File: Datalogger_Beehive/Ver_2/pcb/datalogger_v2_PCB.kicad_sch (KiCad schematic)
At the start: 75 parts, among them U1 DS18B20, U10 DS18B20, U11 DS18B20, U12 DS18B20, U13 DS18B20, U14 DS18B20, U15 DS18B20, U16 DS18B20, U17 DS18B20, U18 DS18B20, U19 DS18B20, U2 DS18B20, U20 DS18B20, U21 DS18B20, U22 DS18B20, U23 DS18B20, U24 DS18B20, U25 DS18B20, U26 DS18B20, U27 DS18B20, U28 DS18B20, U29 DS18B20, U3 DS18B20, U30 DS18B20, U31 DS18B20, U32 DS18B20, U33 DS18B20, U34 DS18B20, U35 DS18B20, U36 DS18B20, U37 DS18B20, U38 DS18B20, U39 DS18B20, U4 DS18B20, U40 DS18B20, U41 DS18B20, U42 DS18B20, U43 DS18B20, U44 DS18B20, U45 DS18B20, U46 DS18B20, U47 DS18B20, U48 DS18B20, U49 DS18B20, U5 DS18B20, U50 DS18B20, U51 DS18B20, U52 DS18B20, U53 DS18B20, U54 DS18B20, U55 DS18B20, U56 DS18B20, U57 DS18B20, U58 DS18B20, U59 DS18B20, U6 DS18B20, U60 DS18B20, U61 DS18B20, U62 DS18B20, U63 DS18B20, U64 DS18B20, U65 DS18B20, U66 DS18B20, U67 DS18B20, U68 DS18B20, U69 DS18B20, U7 DS18B20, U70 DS18B20, U8 DS18B20, U9 DS18B20

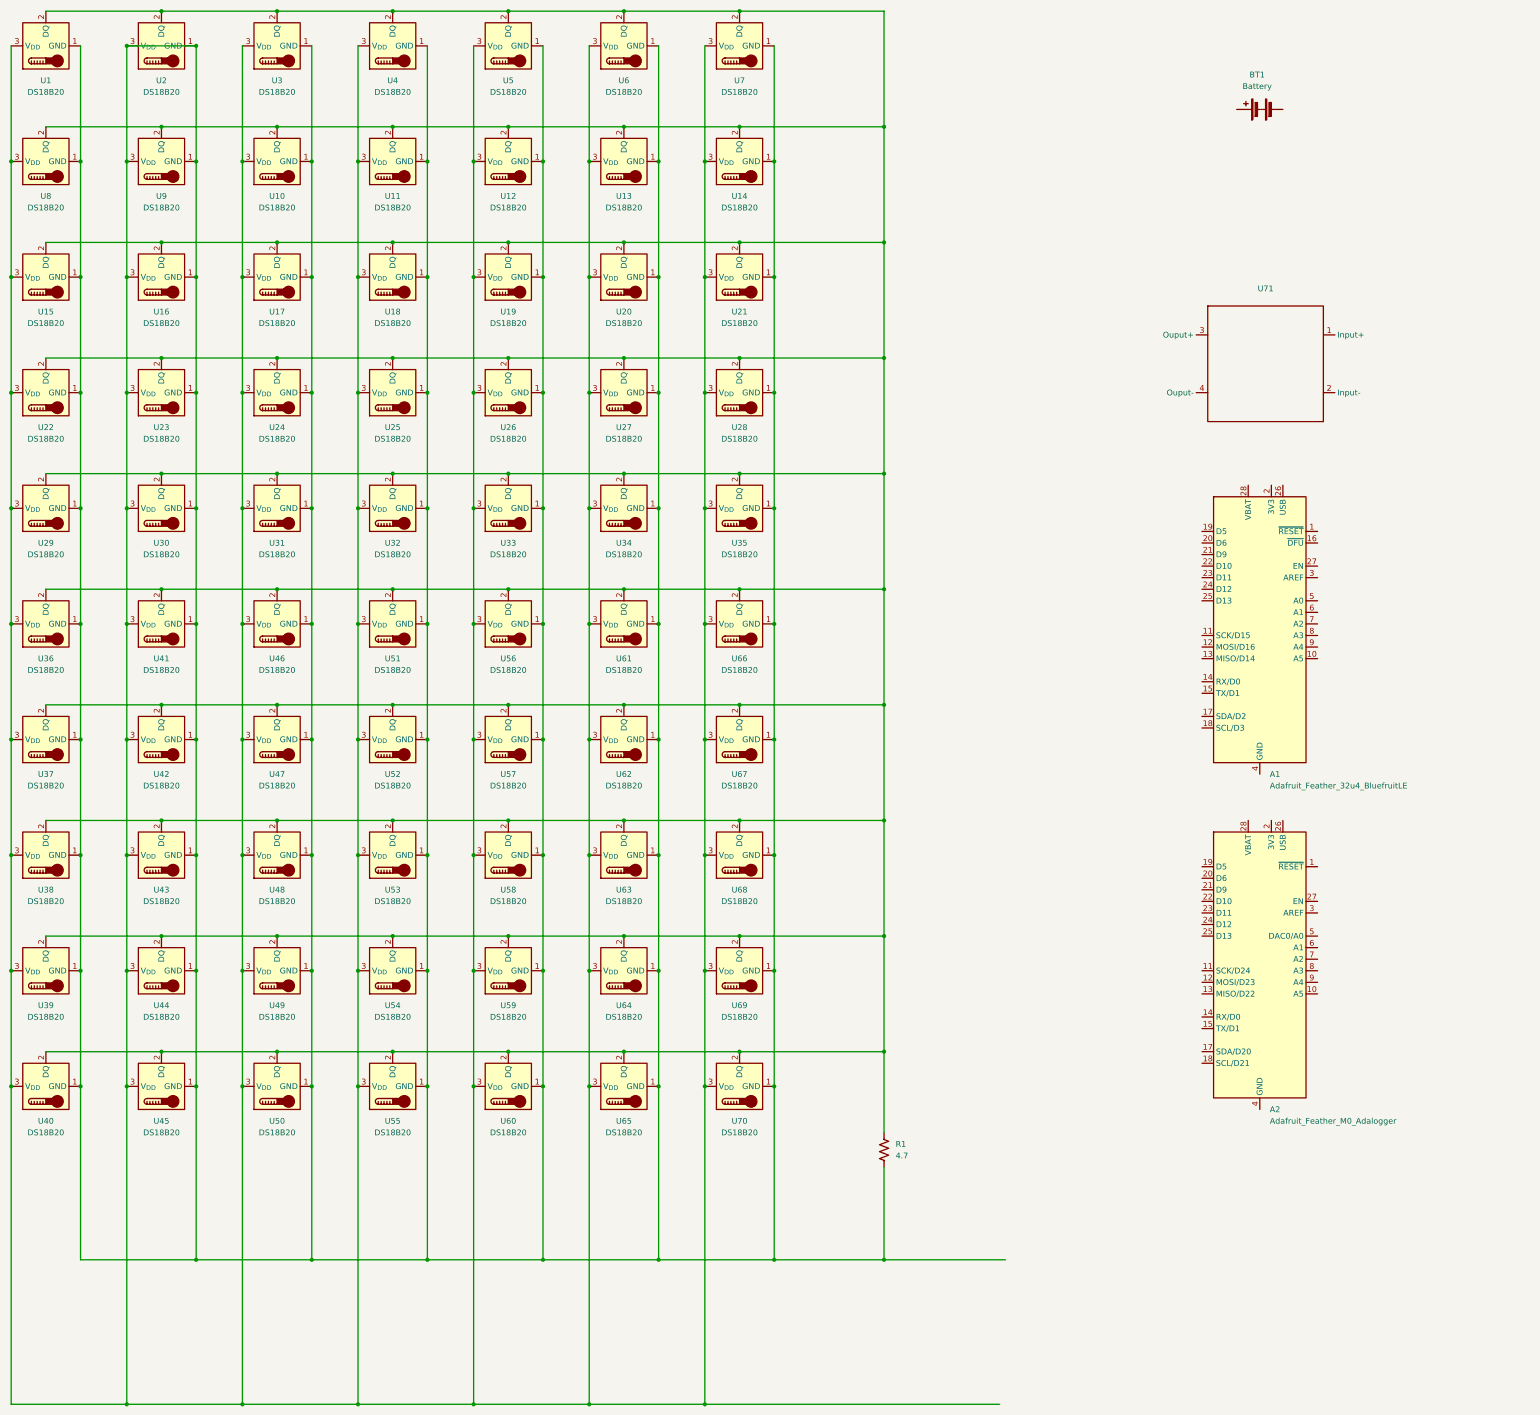
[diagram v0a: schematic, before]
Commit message: enclosure adding
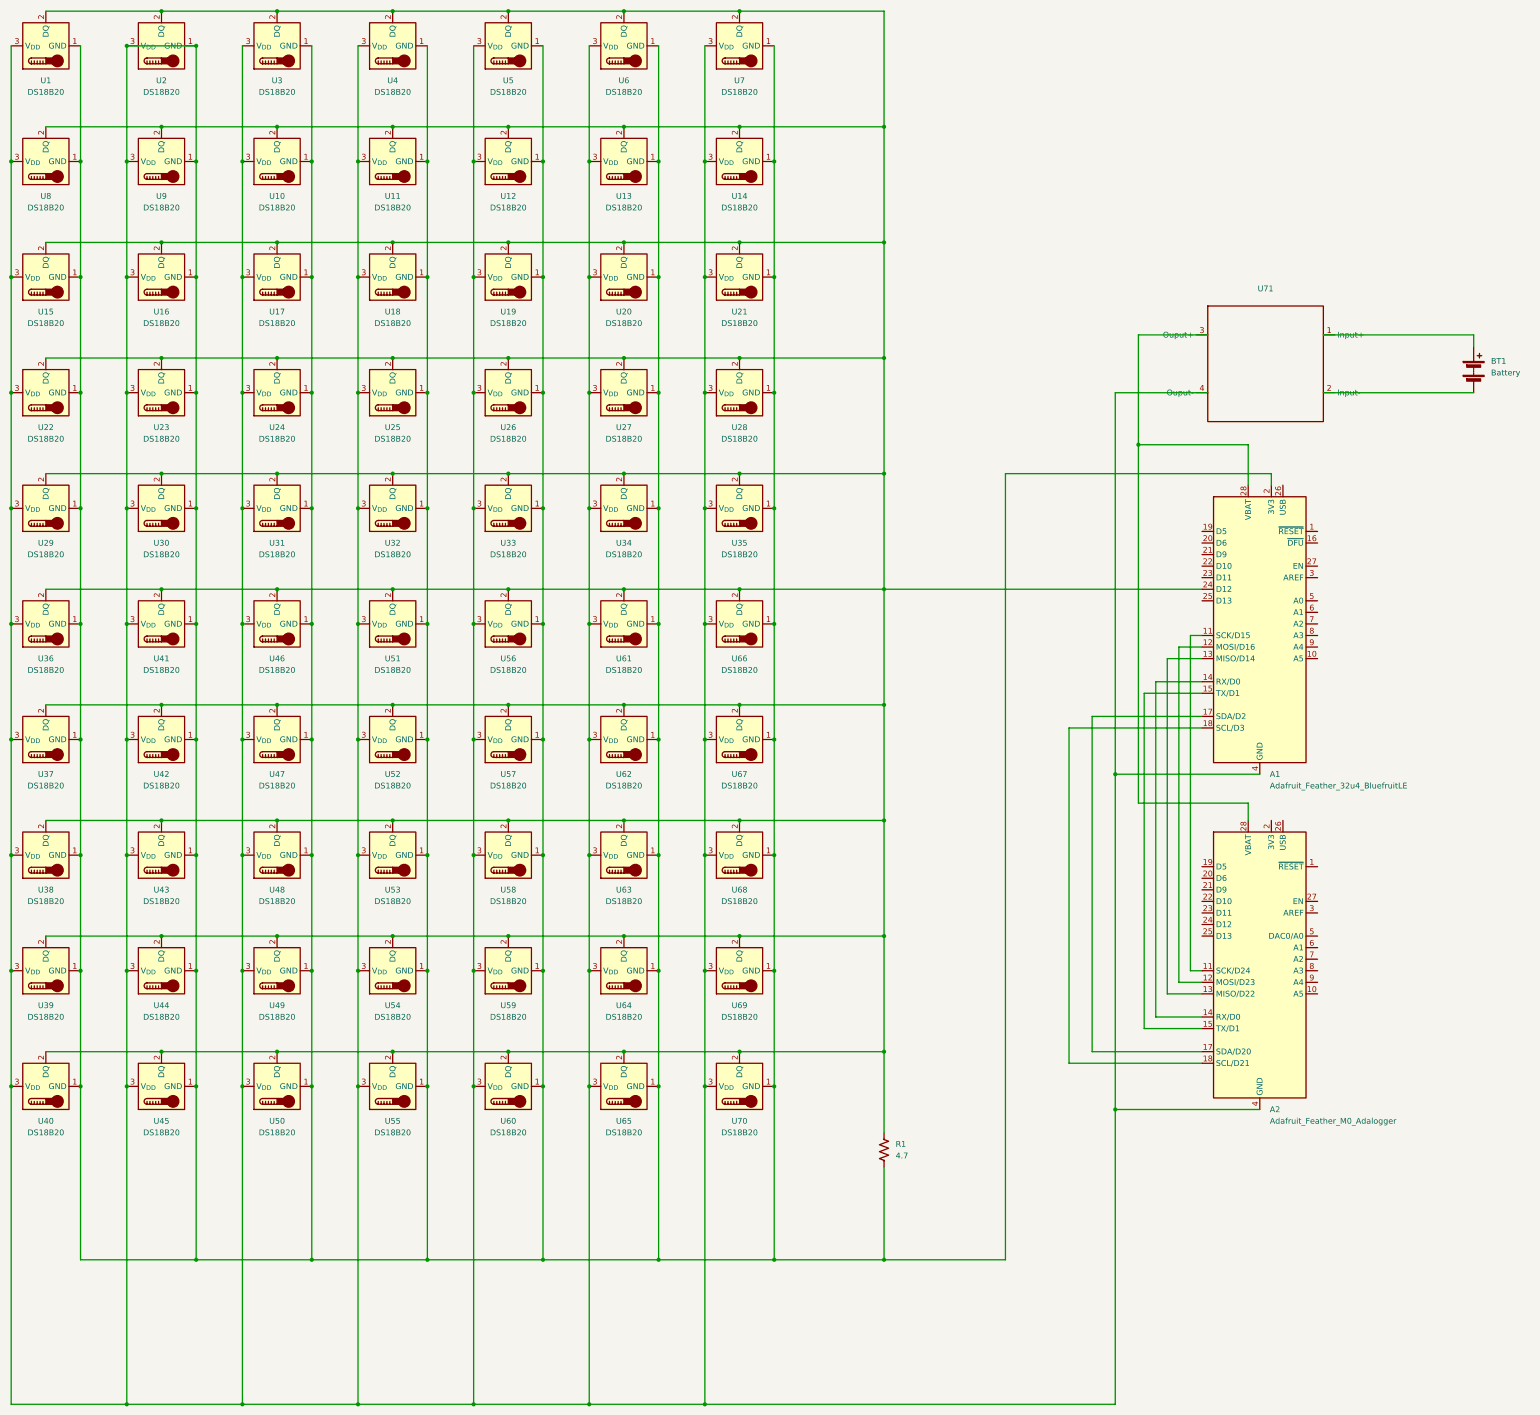
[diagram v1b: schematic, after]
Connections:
- net at R1.2, U1.1 (GND), U1.3 (V_{DD})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: now also A1.2 (3V3), A1.4 (GND), A2.16 (GND), A2.4 (GND), U71.4 (Ouput-)
- net at R1.1, U1.2 (DQ), U10.2 (DQ)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: now also A1.24 (D12)
- net at A1.11 (SCK/D15): now also A2.11 (SCK/D24)
- net at A1.12 (MOSI/D16): now also A2.12 (MOSI/D23)
- net at A1.13 (MISO/D14): now also A2.13 (MISO/D22)
- net at A1.14 (RX/D0): now also A2.14 (RX/D0)
- net at A1.15 (TX/D1): now also A2.15 (TX/D1)
- net at A1.17 (SDA/D2): now also A2.17 (SDA/D20)
- net at A1.18 (SCL/D3): now also A2.18 (SCL/D21)
- net at A1.28 (VBAT): now also A2.28 (VBAT), U71.3 (Ouput+)
- net at U71.1 (Input+): now also BT1.1 (+)
- net at U71.2 (Input-): now also BT1.2 (-)
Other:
- moved on the sheet: BT1
